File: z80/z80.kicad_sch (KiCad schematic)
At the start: 102 parts, among them J1 PinHeader_Female01x02, J2 PinHeader_Female16x02, J3 PinHeader_Female16x02, J4 PinHeader_Female04x02, J5 PinHeader_Female04x02, J6 PinHeader_Female04x02, J7 PinHeader_Female04x02, J8 PinHeader_Female04x02, J9 PinHeader_Female04x02, SW1 SW_Push, SW2 SW_SP3T, SW3 SW_Push, U1 4081, U10 82C55A, U2 74HC595, U3 74HC595, U4 SN74HC138N, U5 SN74HC138N, U6 4069, U7 82C55A, U8 4081, U9 74LS32

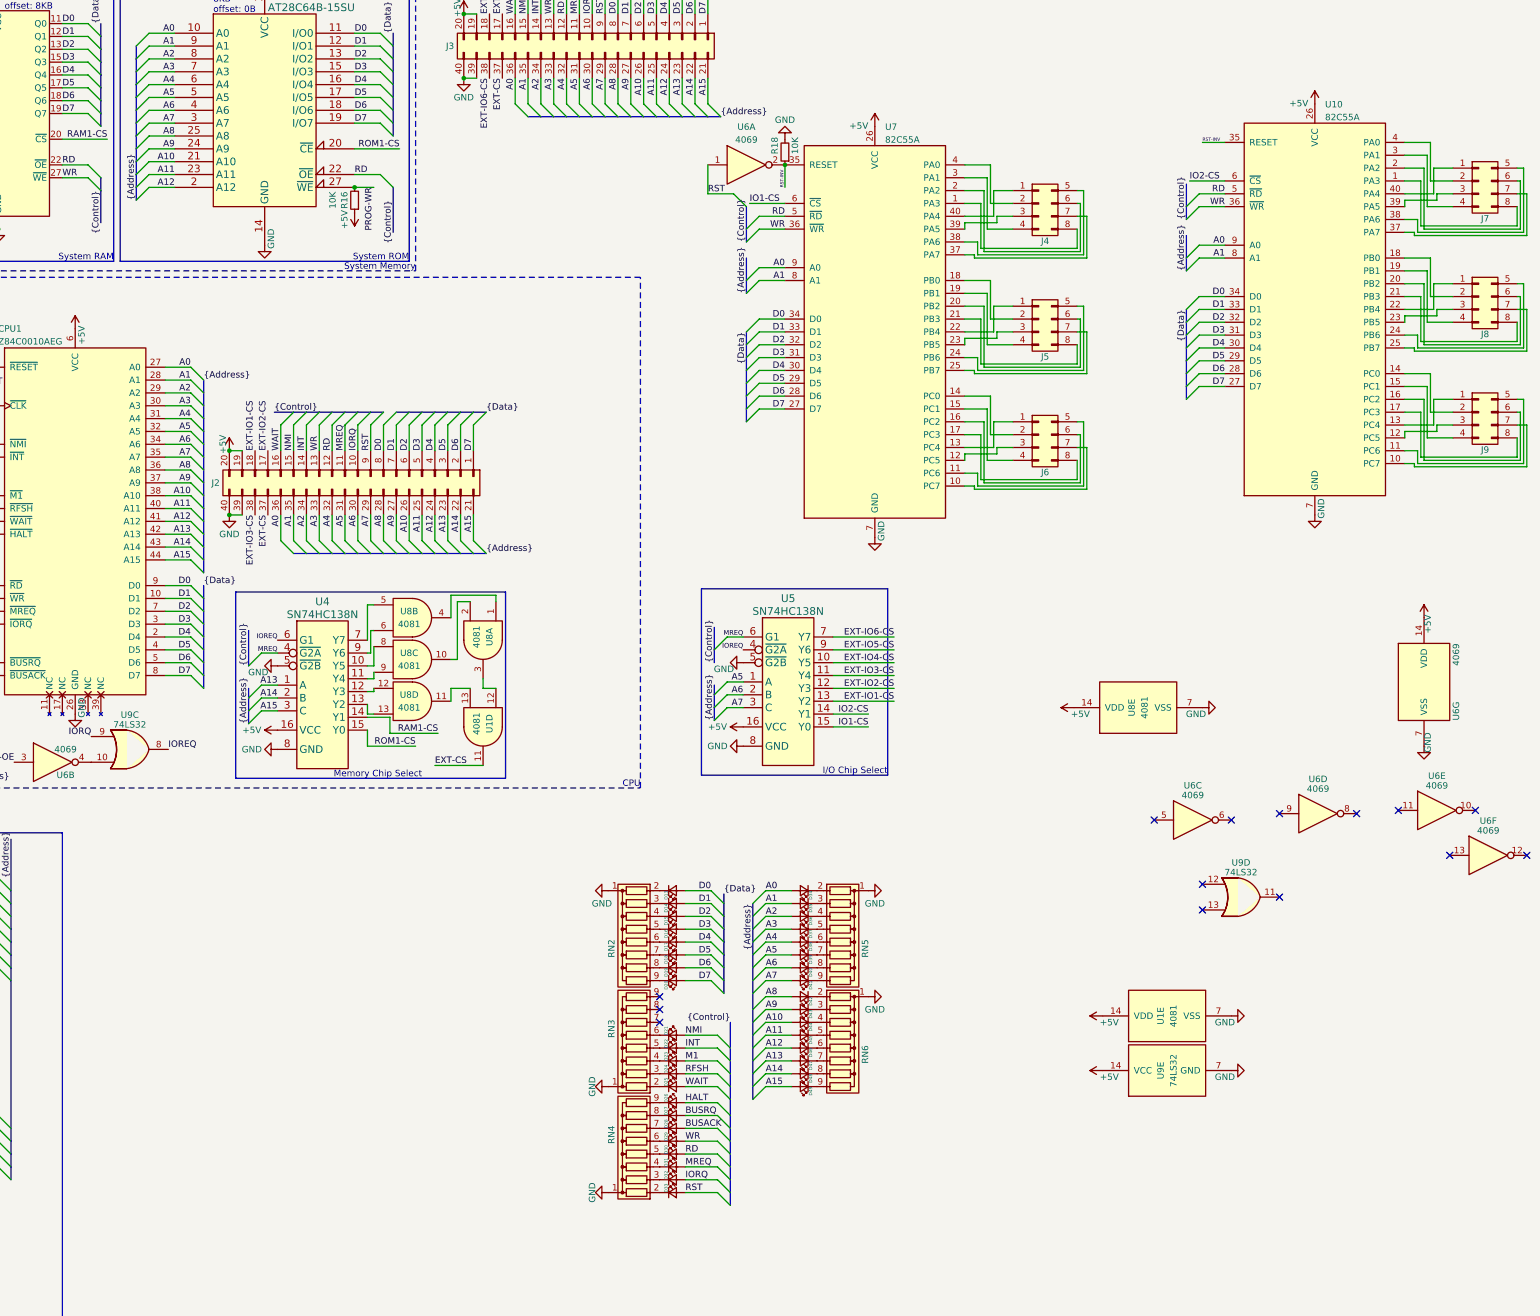
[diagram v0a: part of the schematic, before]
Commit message: Board revision 1
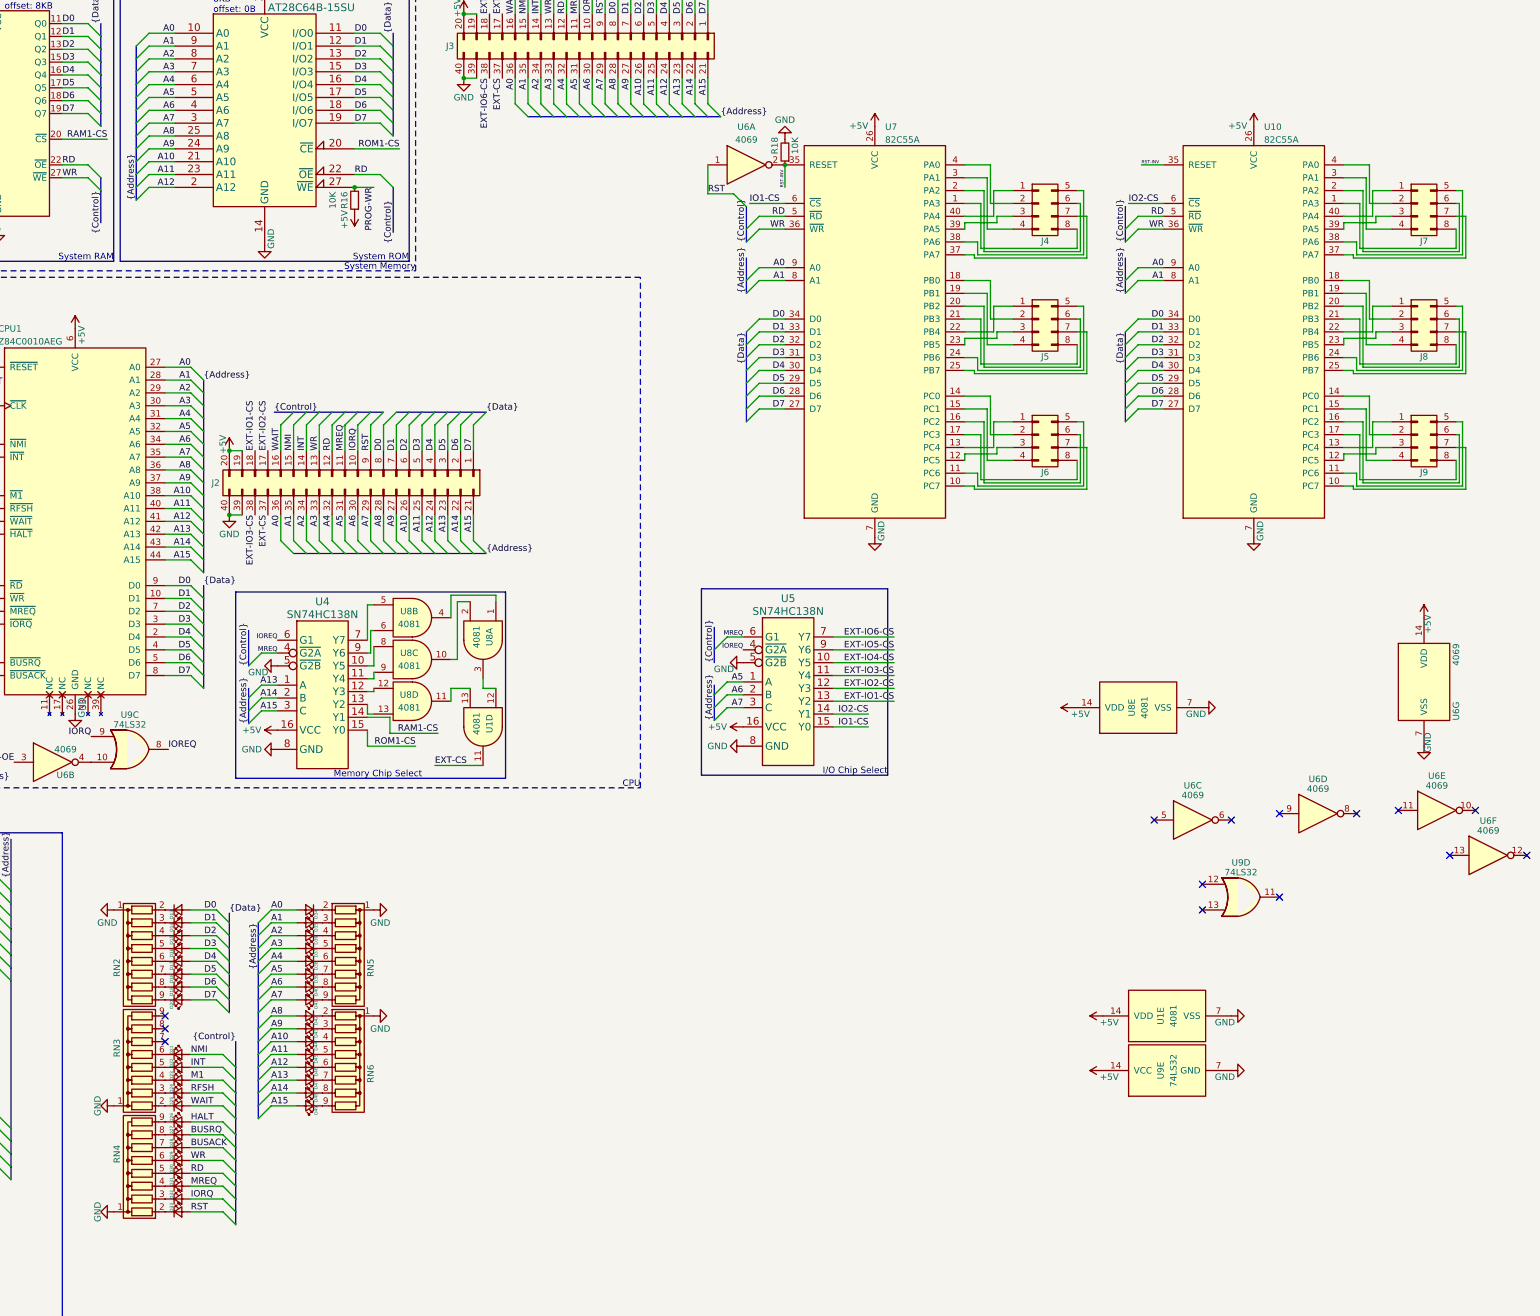
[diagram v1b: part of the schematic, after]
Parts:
- A1: footprint (none) -> Package_DIP:DIP-24_W15.24mm_Socket
- U9: footprint Capacitor_SMD:C_1206_3216Metric -> Package_SO:SOIC-14_3.9x8.7mm_P1.27mm
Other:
- moved on the sheet: D13, D14, D15, D16, D17, D18, D19, D20, D21, D22, D23, D24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
